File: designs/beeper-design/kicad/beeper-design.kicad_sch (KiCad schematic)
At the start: 0 parts

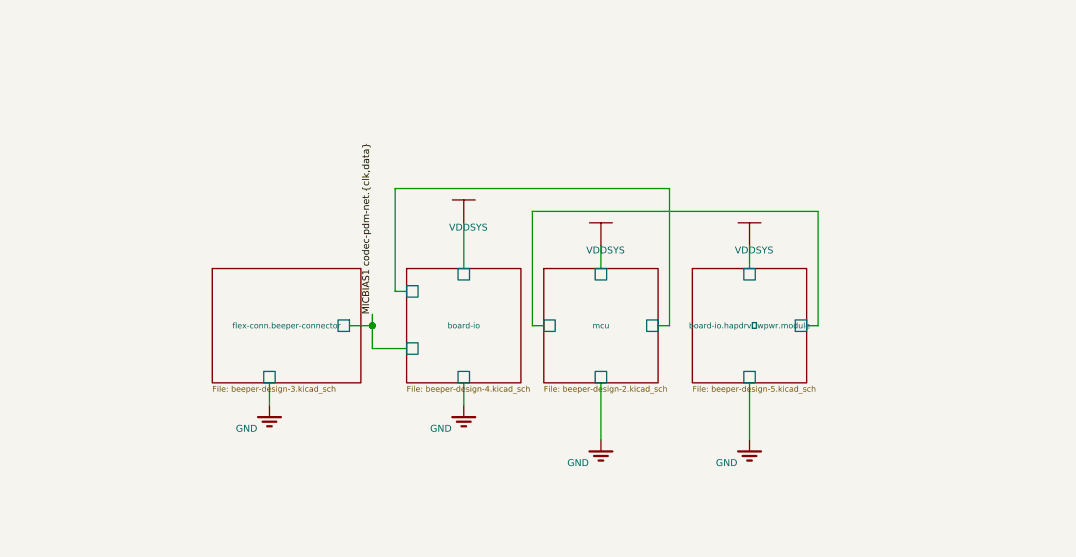
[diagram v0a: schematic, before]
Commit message: kicad exported data
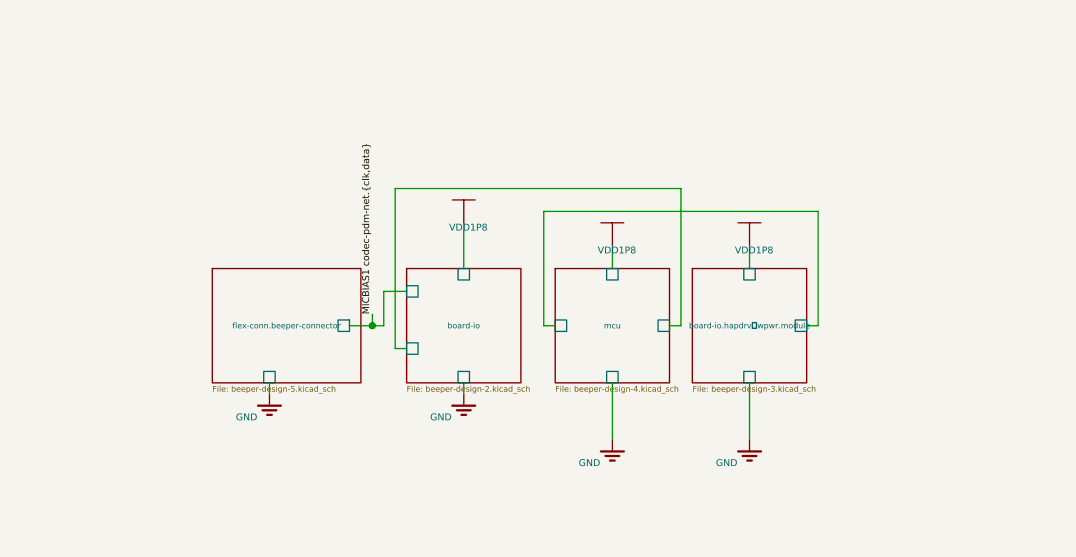
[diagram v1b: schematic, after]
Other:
- sheet board-io: file beeper-design-4.kicad_sch -> beeper-design-2.kicad_sch
- sheet board-io.hapdrv wpwr.module: file beeper-design-5.kicad_sch -> beeper-design-3.kicad_sch
- sheet flex-conn.beeper-connector: file beeper-design-3.kicad_sch -> beeper-design-5.kicad_sch
- sheet mcu: file beeper-design-2.kicad_sch -> beeper-design-4.kicad_sch

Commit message: another export
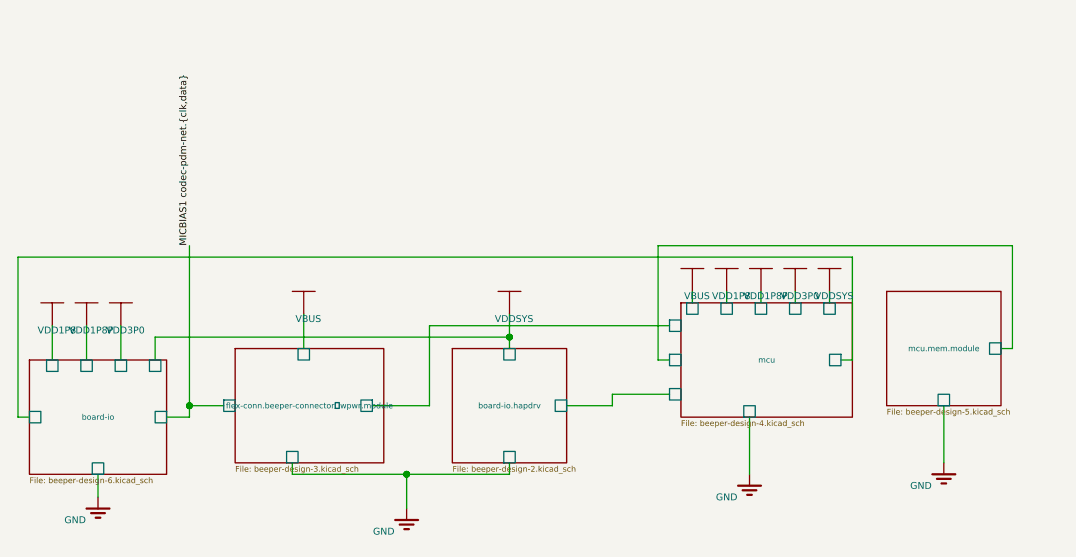
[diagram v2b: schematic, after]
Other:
- removed sheet board-io.hapdrv wpwr.module
- removed sheet flex-conn.beeper-connector
- added sheet board-io.hapdrv (beeper-design-2.kicad_sch)
- added sheet flex-conn.beeper-connector wpwr.module (beeper-design-3.kicad_sch)
- added sheet mcu.mem.module (beeper-design-5.kicad_sch)
- sheet board-io: file beeper-design-2.kicad_sch -> beeper-design-6.kicad_sch
